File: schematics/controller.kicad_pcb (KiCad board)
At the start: 2 copper layers, 21 parts, among them IC1 ESP32-SOLO-1, J1 Conn_01x02, J2 Conn_01x06, J3 Conn_01x09, SW1 SW_Push, SW2 SW_SPDT, SW3 SW_Push_Dual, SW4 SW_Push_Dual, SW5 SW_Push_Dual, SW6 SW_Push_Dual, SW7 SW_Push_Dual, U1 NCP1117-3.3_SOT223

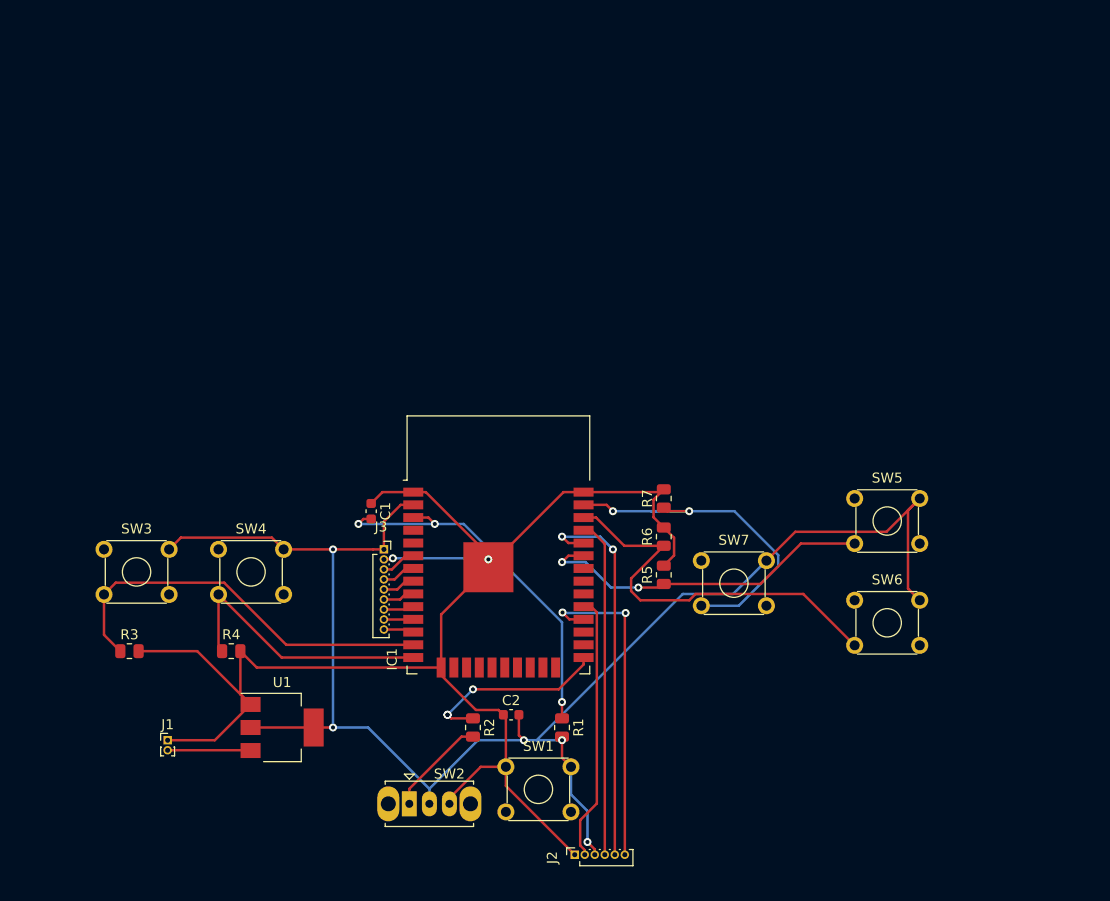
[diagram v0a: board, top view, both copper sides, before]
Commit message: tower pcb
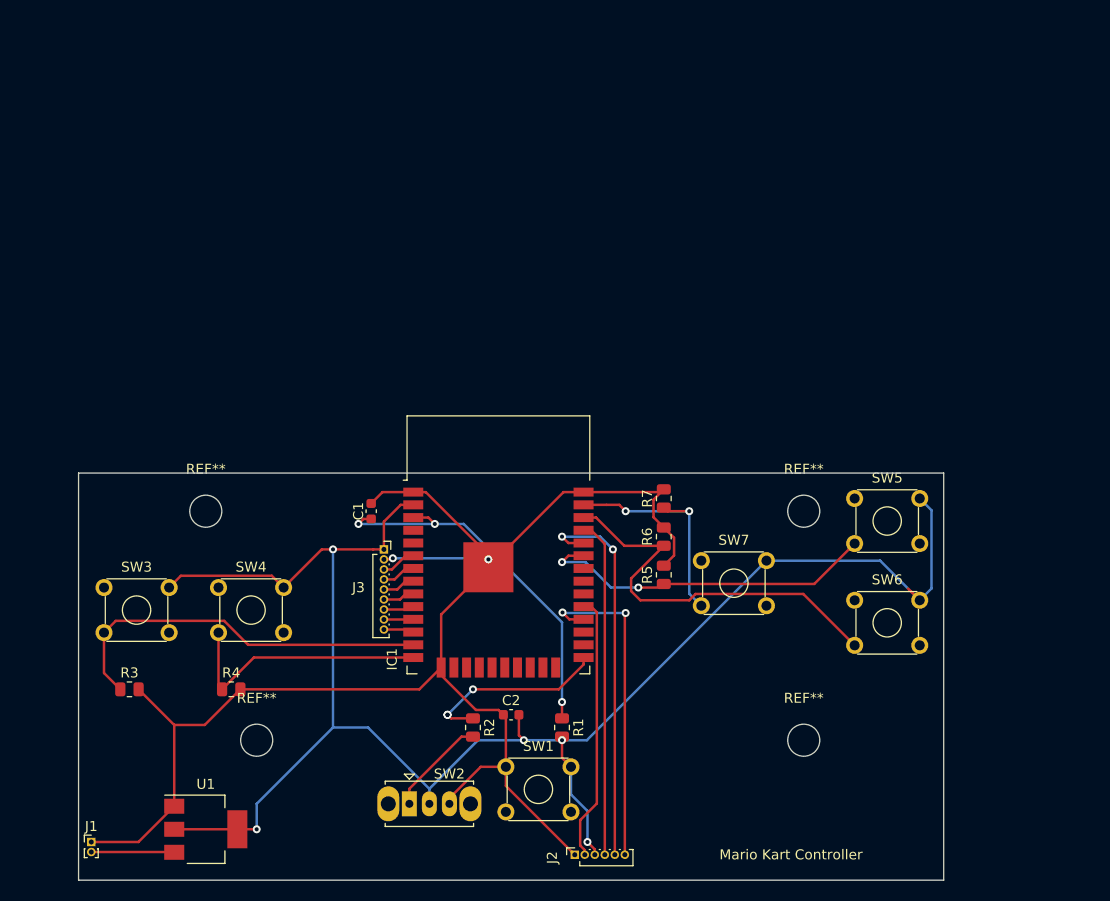
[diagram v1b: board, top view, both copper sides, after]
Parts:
- added REF**: MountingHole_3.2mm_M3, MountingHole:MountingHole_3.2mm_M3, F.Cu at (106.7, 120.7)
- added REF**: MountingHole_3.2mm_M3, MountingHole:MountingHole_3.2mm_M3, F.Cu at (101.6, 97.8)
- added REF**: MountingHole_3.2mm_M3, MountingHole:MountingHole_3.2mm_M3, F.Cu at (161.3, 97.8)
- added REF**: MountingHole_3.2mm_M3, MountingHole:MountingHole_3.2mm_M3, F.Cu at (161.3, 120.7)
- moved J1 12.7 mm to (90.2, 130.8)
- moved U1 12.7 mm to (101.6, 129.5)
- moved SW3 3.81 mm to (91.4, 105.4)
- moved SW4 3.81 mm to (102.9, 105.4)
- moved R3 3.81 mm to (94.0, 115.6)
- moved R4 3.81 mm to (104.1, 115.6)
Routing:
- net Net-(IC1-Pad37): track 38.4 -> 23.4 mm
- net Vcc: track 159.7 -> 172.8 mm
- net GND: track 152.4 -> 154.7 mm
- net S4: track 27.9 -> 26.2 mm
- net S3: track 40.3 -> 38.7 mm
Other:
- board outline added: 86.4 x 40.6 mm
- board text added: "Mario Kart Controller"

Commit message: finished (I think) schematics for tower and controller
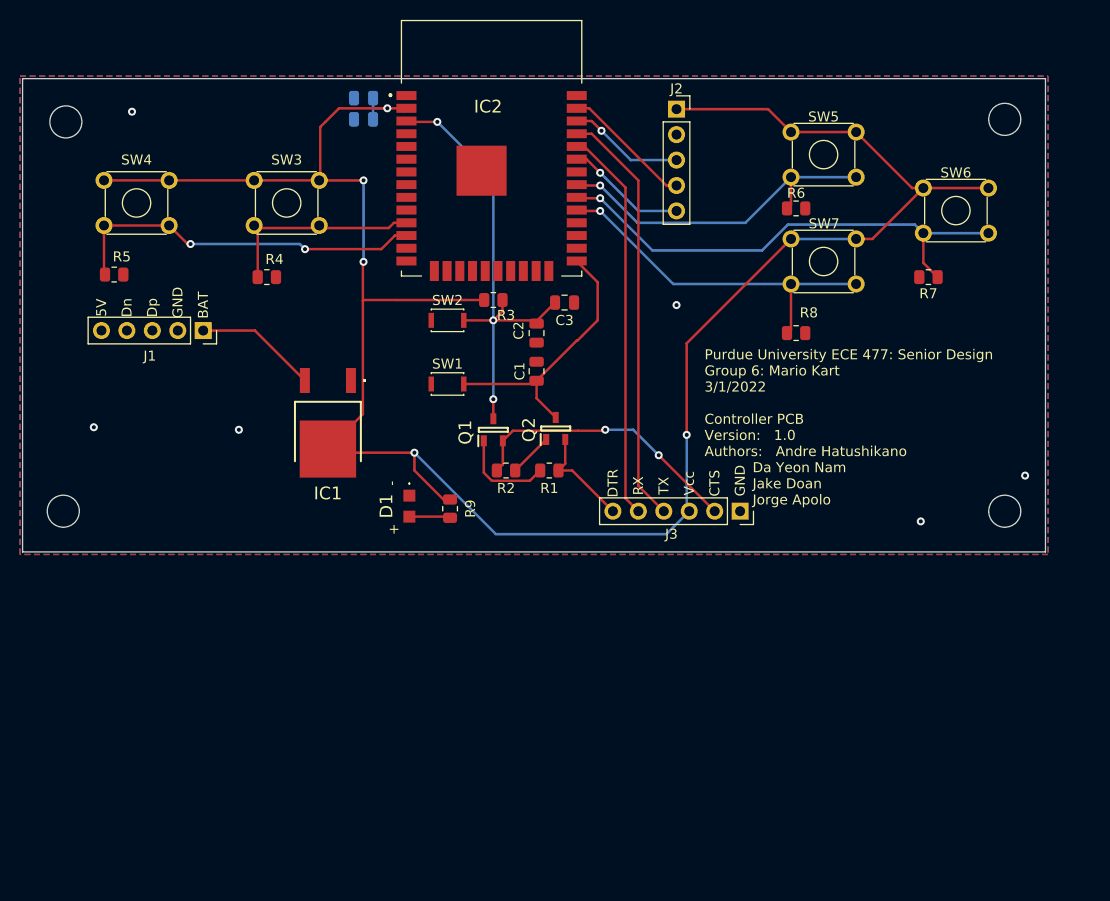
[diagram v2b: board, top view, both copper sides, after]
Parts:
- removed the REF** at (106.7, 120.7)
- removed the REF** at (101.6, 97.8)
- removed the REF** at (161.3, 97.8)
- removed the REF** at (161.3, 120.7)
- removed U1: NCP1117-3.3_SOT223, Package_TO_SOT_SMD:SOT-223-3_TabPin2
- added C3: 100nF, Capacitor_SMD:C_0805_2012Metric, F.Cu at (137.4, 77.0)
- added C4: 22uF, Capacitor_SMD:C_0805_2012Metric, B.Cu at (117.3, 56.6)
- added C5: 100nF, Capacitor_SMD:C_0805_2012Metric, B.Cu at (117.3, 58.7)
- added D1: LED, Mouser:APHCM2012QBCDF01, F.Cu at (121.9, 97.3)
- added IC2: ESP32-SOLO-1, Mouser:ESP32SOLO1, F.Cu at (130.1, 61.8)
- added Q1: SS8050-G, Mouser:SOT95P240X115-3N, F.Cu at (130.3, 89.7)
- added Q2: SS8050-G, Mouser:SOT95P240X115-3N, F.Cu at (136.5, 89.5)
- added R8: 10k, Resistor_SMD:R_0805_2012Metric, F.Cu at (160.5, 80.0)
- added R9: 0, Resistor_SMD:R_0805_2012Metric, F.Cu at (126.0, 97.5)
- added REF**: MountingHole_3.2mm_M3, MountingHole:MountingHole_3.2mm_M3, F.Cu at (87.4, 97.8)
- added REF**: MountingHole_3.2mm_M3, MountingHole:MountingHole_3.2mm_M3, F.Cu at (87.6, 58.9)
- added REF**: MountingHole_3.2mm_M3, MountingHole:MountingHole_3.2mm_M3, F.Cu at (181.4, 58.7)
- added REF**: MountingHole_3.2mm_M3, MountingHole:MountingHole_3.2mm_M3, F.Cu at (181.4, 97.8)
- C1, C2: value 100nF -> 0.1uF; footprint Capacitor_SMD:C_0603_1608Metric -> Capacitor_SMD:C_0805_2012Metric
- IC1: value ESP32-SOLO-1 -> AZ1117CD-3.3TRG1; footprint RF_Module:ESP32-WROOM-32 -> Mouser:AZ1117CD33TRG1
- J1: value Conn_01x02 -> Conn_01x05; footprint Connector_PinHeader_1.00mm:PinHeader_1x02_P1.00mm_Vertical -> Connector_PinSocket_2.54mm:PinSocket_1x05_P2.54mm_Vertical
- J2: value Conn_01x06 -> Conn_01x05; footprint Connector_PinSocket_1.00mm:PinSocket_1x06_P1.00mm_Vertical -> Connector_PinSocket_2.54mm:PinSocket_1x05_P2.54mm_Vertical
- J3: value Conn_01x09 -> Conn_01x06; footprint Connector_PinSocket_1.00mm:PinSocket_1x09_P1.00mm_Vertical -> Connector_PinSocket_2.54mm:PinSocket_1x06_P2.54mm_Vertical
- SW1: footprint Button_Switch_THT:SW_TH_Tactile_Omron_B3F-10xx -> Button_Switch_SMD:SW_SPST_CK_KXT3
- SW2: value SW_SPDT -> SW_Push; footprint Button_Switch_THT:SW_Slide_1P2T_CK_OS102011MS2Q -> Button_Switch_SMD:SW_SPST_CK_KXT3
- moved J2 75.1 mm to (148.6, 57.7), turned to 0 degrees
- moved R5 62.5 mm to (92.5, 74.2), turned to 0 degrees
- moved R3 53.2 mm to (130.3, 76.7)
- moved J1 52.3 mm to (101.3, 79.8), turned to 270 degrees
- moved SW2 48.4 mm to (125.7, 78.7)
- moved SW3 43.3 mm to (106.4, 64.8)
- moved SW4 42.2 mm to (91.4, 64.8)
- moved SW6 41.7 mm to (173.2, 65.5)
- moved R4 41.3 mm to (107.7, 74.4)
- moved SW1 38.7 mm to (125.7, 85.1)
- moved C2 38.2 mm to (134.6, 80.0), turned to 270 degrees
- moved SW5 37.1 mm to (160.0, 59.9)
- moved J3 35.8 mm to (154.9, 97.8), turned to 270 degrees
- moved R6 35.3 mm to (160.5, 67.6), turned to 0 degrees
- moved R7 34.4 mm to (173.7, 74.4), turned to 180 degrees
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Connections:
- C1 pad 1: GND -> GPIO0
- C1 pad 2: Net-(C1-Pad2) -> GND
- C2 pad 1: GND -> EN
- C2 pad 2: Vcc -> GND
- IC1 pad 3: Net-(C1-Pad2) -> BAT
- J1 pad 1: GND -> BAT
- J1 pad 2: 5V -> GND
- J2 pad 1: GND -> Vcc
- J2 pad 2: CTS -> GND
- J2 pad 3: Vcc -> GPIO22
- J2 pad 4: TX -> GPIO23
- J2 pad 5: RX -> GPIO13
- J3 pad 1: Vcc -> GND
- J3 pad 2: GND -> CTS
- J3 pad 3: IO34 -> Vcc
- J3 pad 4: IO35 -> TX
- J3 pad 5: IO32 -> RX
- J3 pad 6: IO33 -> DTR
- R1 pad 1: Net-(C1-Pad2) -> DTR
- R1 pad 2: Vcc -> Net-(Q1-Pad1)
- R2 pad 1: Net-(IC1-Pad25) -> CTS
- R2 pad 2: Net-(R2-Pad2) -> Net-(Q2-Pad1)
- R3 pad 1: S3 -> Vcc
- R3 pad 2: GND -> EN
- R4 pad 1: S4 -> S1
- R5 pad 1: Net-(IC1-Pad33) -> S2
- R6 pad 1: Net-(IC1-Pad36) -> S3
- R7 pad 1: Net-(IC1-Pad37) -> S4
- SW1 pad 2: Vcc -> GPIO0
- SW2 pad 1: Net-(R2-Pad2) -> GND
- SW2 pad 2: Vcc -> EN
- SW3 pad 1: Net-(SW3-Pad1) -> Vcc
- SW3 pad 3: S3 -> S1
- SW3 pad 4: Net-(SW3-Pad4) -> S1
- SW4 pad 1: Net-(SW4-Pad1) -> Vcc
- SW4 pad 3: S4 -> S2
- SW4 pad 4: Net-(SW4-Pad4) -> S2
- SW5 pad 1: Net-(SW5-Pad1) -> Vcc
- SW5 pad 3: Net-(IC1-Pad33) -> S3
- SW5 pad 4: Net-(SW5-Pad4) -> S3
- SW6 pad 1: Net-(SW6-Pad1) -> Vcc
- SW6 pad 3: Net-(IC1-Pad36) -> S4
- SW6 pad 4: Net-(SW6-Pad4) -> S4
- SW7 pad 1: Net-(SW7-Pad1) -> Vcc
- SW7 pad 3: Net-(IC1-Pad37) -> S5
- SW7 pad 4: Net-(SW7-Pad4) -> S5
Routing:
- net GND: track 154.7 -> 1.05 mm, vias 2 -> 6
- net EN: track 0.00 -> 48.0 mm, vias 0 -> 3
- net Vcc: track 172.8 -> 214.5 mm
- net Net-(IC1-Pad36): track 40.1 -> 0.00 mm
- net Net-(C1-Pad2): track 37.9 -> 0.00 mm, vias 3 -> 0
- net S2: track 0.00 -> 36.9 mm, vias 0 -> 2
- net S5: track 0.00 -> 36.0 mm, vias 0 -> 1
- net Net-(IC1-Pad33): track 34.5 -> 0.00 mm, vias 2 -> 0
- net GPIO0: track 0.00 -> 27.2 mm
- net S4: track 26.2 -> 49.7 mm, vias 0 -> 1
- net Net-(IC1-Pad37): track 23.4 -> 0.00 mm, vias 2 -> 0
- net DTR: track 32.9 -> 10.5 mm, vias 2 -> 0
- net S1: track 0.00 -> 21.6 mm
- net Net-(IC1-Pad25): track 19.0 -> 0.00 mm, vias 3 -> 0
- net GPIO23: track 0.00 -> 13.2 mm
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- added copper zone on B.Cu, net GND
- added copper zone on F.Cu, net GND
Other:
- board size 86.4 x 40.6 mm -> 102.1 x 47.2 mm
- board text added: "+"
- board text added: "-"
- board text added: "5V"
- board text added: "BAT"
- board text added: "CTS"
- board text added: "DTR"
- board text added: "Dn"
- board text added: "Dp"
- board text added: "GND"
- board text added: "Purdue University ECE 477: Senior Design Group 6: Mario Kart 3/1/2022 Controller PCB Version: 1.0 Authors: Andre Hatushikano Da Yeon Nam Jake Doan Jorge Apolo"
- board text added: "RX"
- board text added: "TX"
- board text added: "Vcc"
- board text removed: "Mario Kart Controller"

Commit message: converted all schematics into kicad6 format
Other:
- net class Default removed
